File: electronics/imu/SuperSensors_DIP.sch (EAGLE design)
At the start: 11 parts, among them J2 AVR_SPI_PRG_6PTH, U1 ATMEGA328P-AU

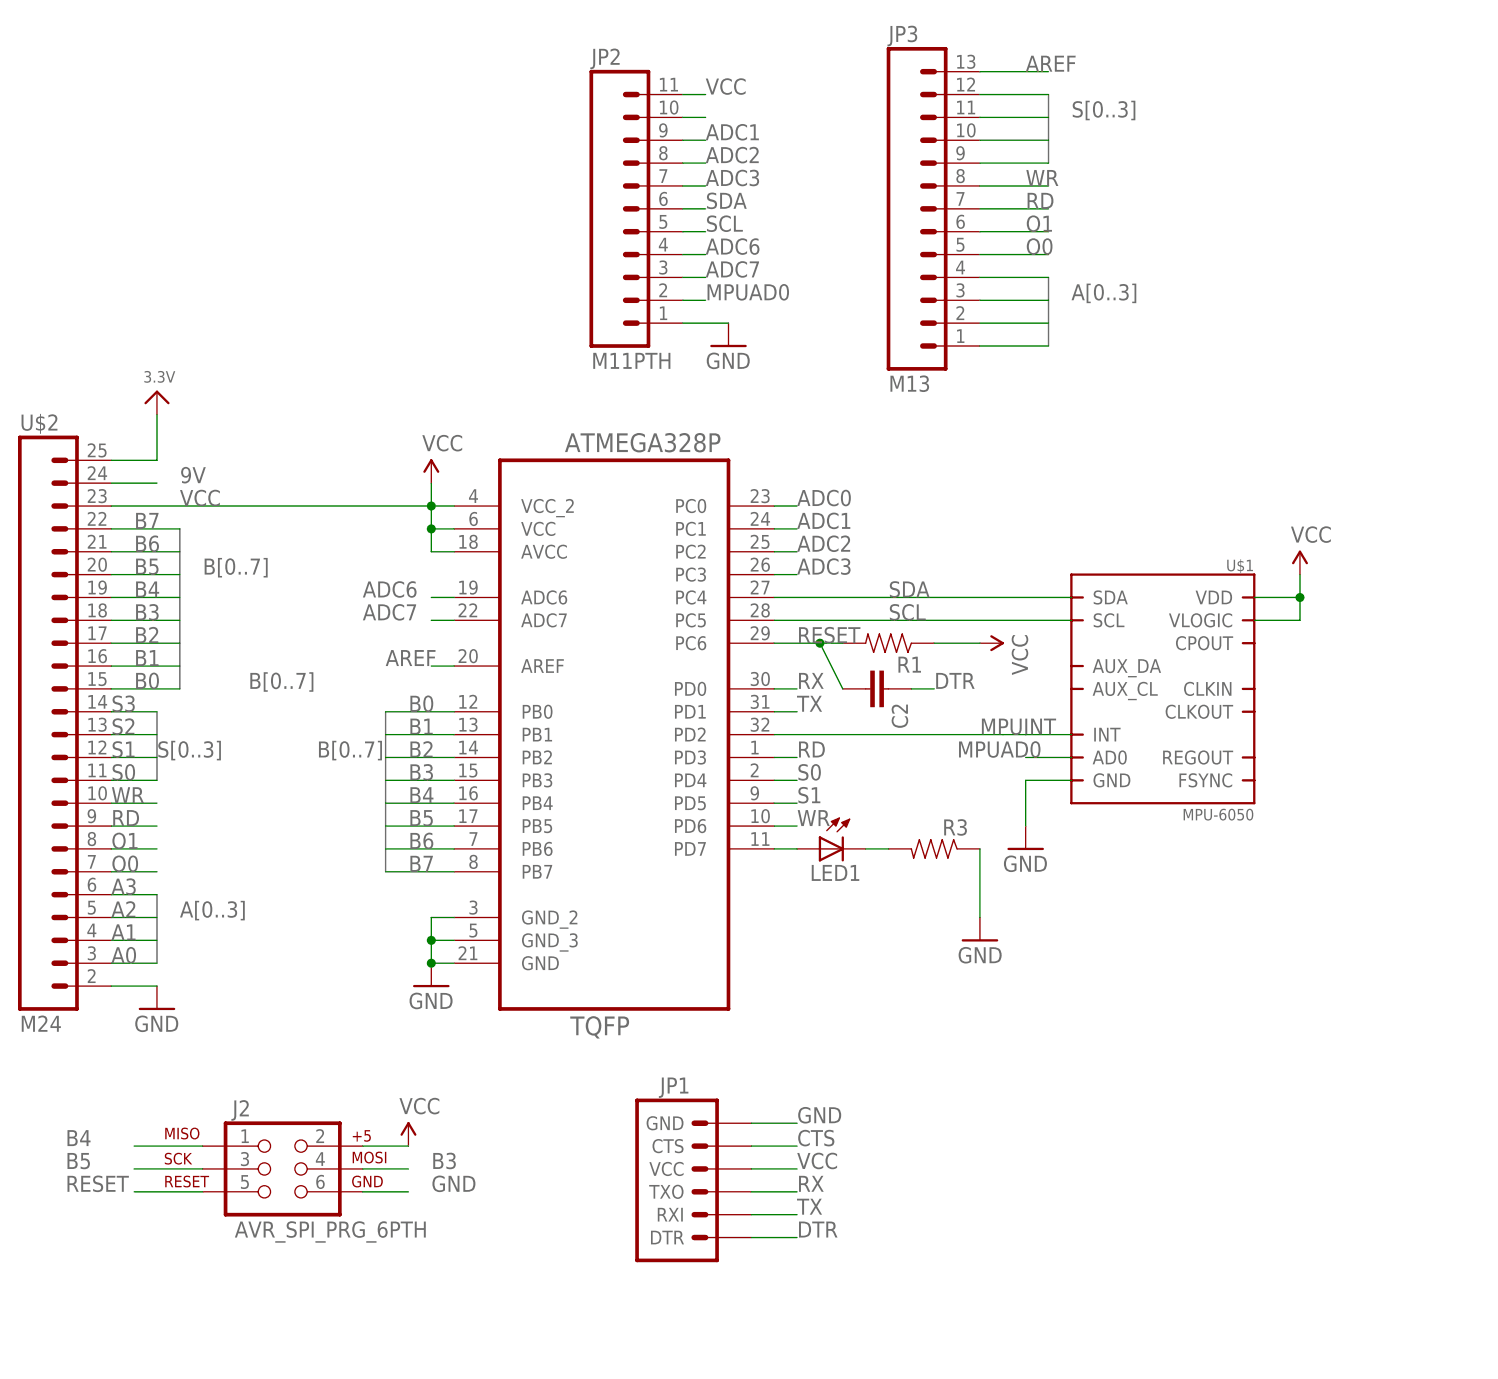
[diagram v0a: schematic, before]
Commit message: board layout
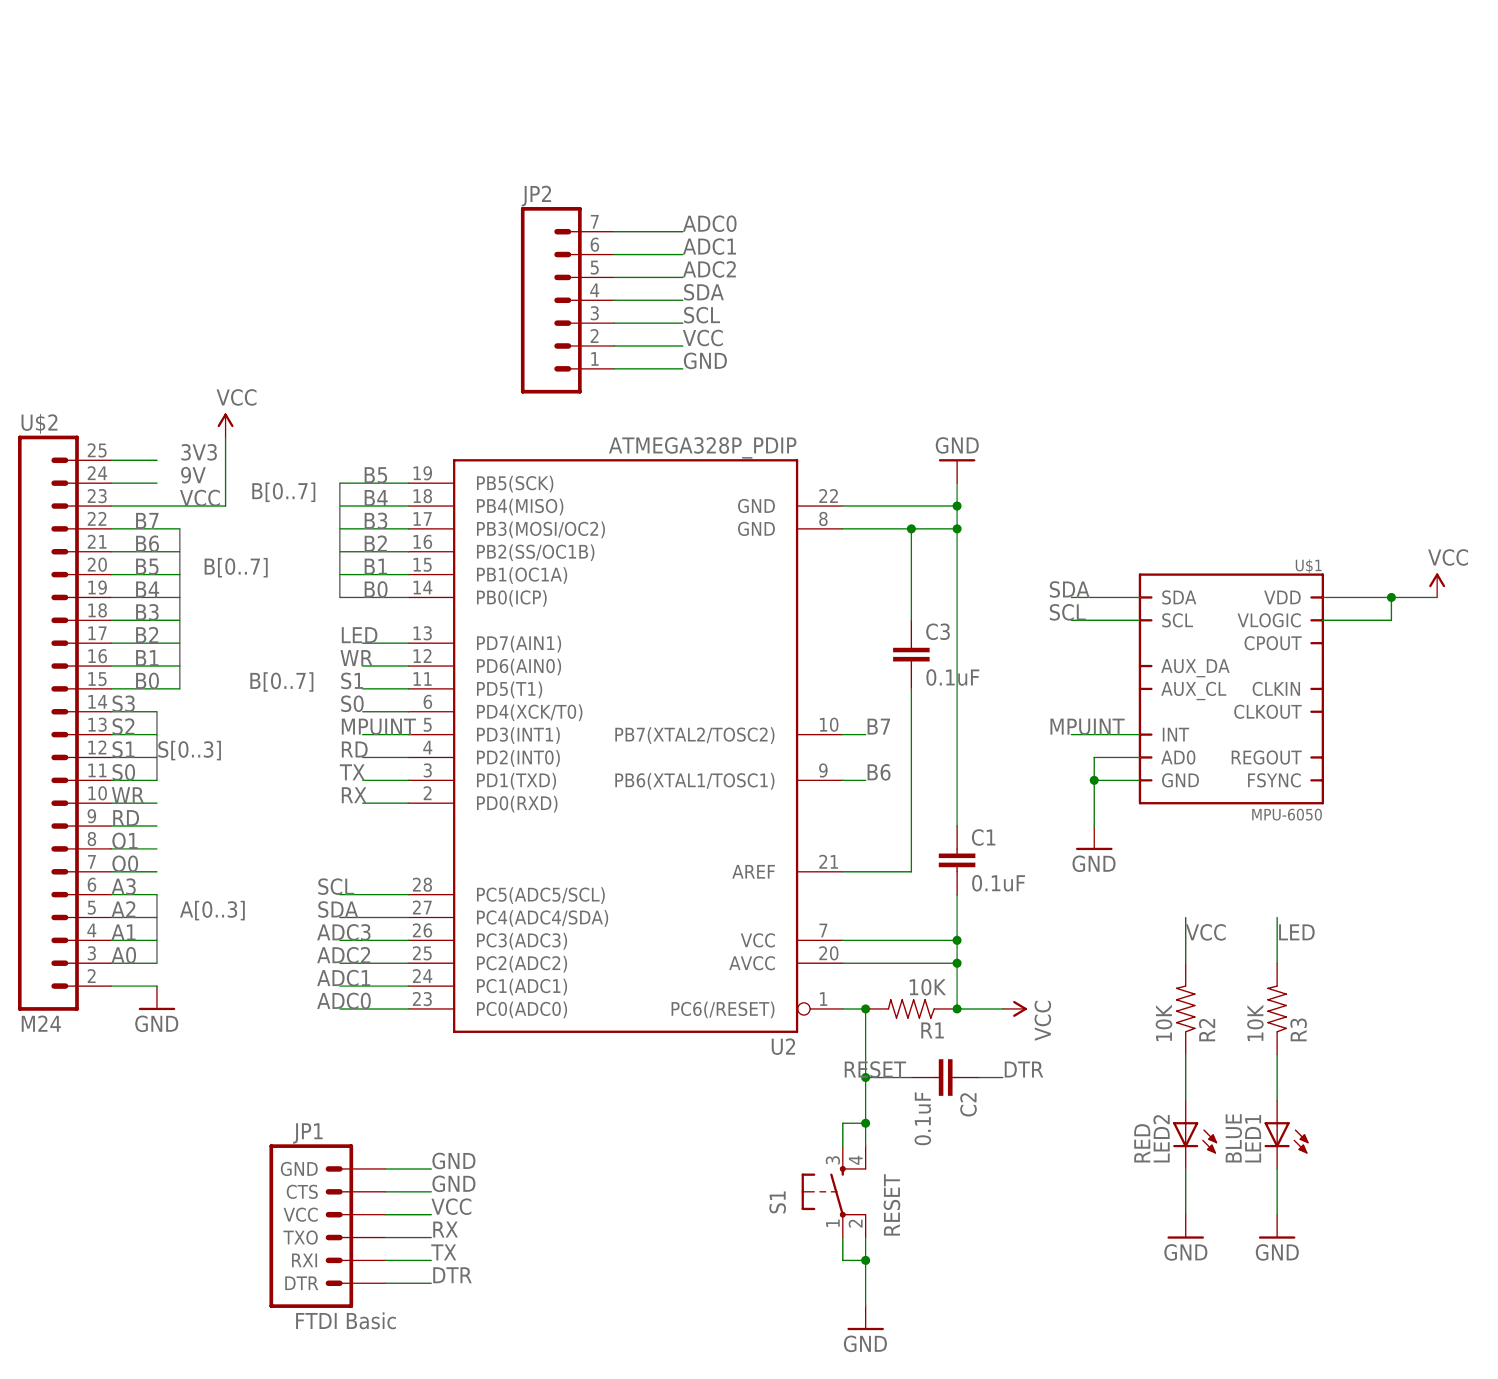
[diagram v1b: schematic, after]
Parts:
- removed J2: AVR_SPI_PRG_6PTH, SparkFun-Connectors:AVR_SPI_PRG_6PTH
- removed JP3: M13, SparkFun-Connectors:M13
- removed U1: ATMEGA328P-AU, Ava:ATMEGA328P-AU
- added C1, C3: 0.1uF, SparkFun-Capacitors:CAPPTH
- added LED2: RED, SparkFun-LED:LED5MM
- added R2: 10K, SparkFun-Passives:RESISTORPTH-1/4W
- added S1: RESET, SparkFun-Electromechanical:TAC_SWITCHSMD
- added U2: ATMEGA328P_PDIP, SparkFun-DigitalIC:ATMEGA328P_PDIP
- C2: value (none) -> 0.1uF
- JP1: value (none) -> FTDI Basic
- JP2: value M11PTH -> (none); device SparkFun-Connectors:M11PTH -> SparkFun-Connectors:M07
- LED1: value (none) -> BLUE
- R1, R3: value (none) -> 10K
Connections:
- net 3.3V renamed 3V3
- removed net ADC6: JP2.4, U1.ADC6
- removed net ADC7: JP2.3, U1.ADC7
- removed net AREF: JP3.13, U1.AREF
- removed net CTS: JP1.CTS
- removed net MPUAD0: JP2.2, U$1.AD0
- removed net N$5: LED1.C, R3.2
- new net LED: R3.2, U2.PD7(AIN1)
- new net N$2: C3.2, U2.AREF
- new net N$3: LED1.A, R3.1
- net A0: no longer JP3.1
- net A1: no longer JP3.2
- net A2: no longer JP3.3
- net A3: no longer JP3.4
- net ADC0: now also JP2.7, U2.PC0(ADC0); no longer JP2.10, U1.PC0
- net ADC1: now also JP2.6, U2.PC1(ADC1); no longer JP2.9, U1.PC1
- net ADC2: now also JP2.5, U2.PC2(ADC2); no longer JP2.8, U1.PC2
- net ADC3: now also U2.PC3(ADC3); no longer JP2.7, U1.PC3
- net B0: now also U2.PB0(ICP); no longer U1.PB0
- net B1: now also U2.PB1(OC1A); no longer U1.PB1
- net B2: now also U2.PB2(SS/OC1B); no longer U1.PB2
- net B3: now also U2.PB3(MOSI/OC2); no longer J2.4, U1.PB3
- net B4: now also U2.PB4(MISO); no longer J2.1, U1.PB4
- net B5: now also U2.PB5(SCK); no longer J2.3, U1.PB5
- net B6: now also U2.PB6(XTAL1/TOSC1); no longer U1.PB6
- net B7: now also U2.PB7(XTAL2/TOSC2); no longer U1.PB7
- net GND: now also C1.1, C3.1, JP1.CTS, LED1.C, LED2.C, S1.1, S1.2, U$1.AD0, U2.GND@1, U2.GND@2; no longer J2.6, R3.1, U1.GND, U1.GND_2, U1.GND_3
- net MPUINT: now also U2.PD3(INT1); no longer U1.PD2
- net N$1: now also LED2.A, R2.1; no longer LED1.A, U1.PD7
- net O0: no longer JP3.5
- net O1: no longer JP3.6
- net RD: now also U2.PD2(INT0); no longer JP3.7, U1.PD3
- net RESET: now also S1.3, S1.4, U2.PC6(/RESET); no longer J2.5, U1.PC6
- net RX: now also U2.PD0(RXD); no longer U1.PD0
- net S0: now also U2.PD4(XCK/T0); no longer JP3.9, U1.PD4
- net S1: now also U2.PD5(T1); no longer JP3.10, U1.PD5
- net S2: no longer JP3.11
- net S3: no longer JP3.12
- net SCL: now also JP2.3, U2.PC5(ADC5/SCL); no longer JP2.5, U1.PC5
- net SDA: now also JP2.4, U2.PC4(ADC4/SDA); no longer JP2.6, U1.PC4
- net TX: now also U2.PD1(TXD); no longer U1.PD1
- net VCC: now also C1.2, JP2.2, R2.2, U2.AVCC, U2.VCC; no longer J2.2, JP2.11, U1.AVCC, U1.VCC, U1.VCC_2
- net WR: now also U2.PD6(AIN0); no longer JP3.8, U1.PD6
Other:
- moved on the sheet: C2, JP1, LED1, R1, R3, U$1
